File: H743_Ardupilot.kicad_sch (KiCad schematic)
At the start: 8 parts, among them U1 USBLC6-2P6

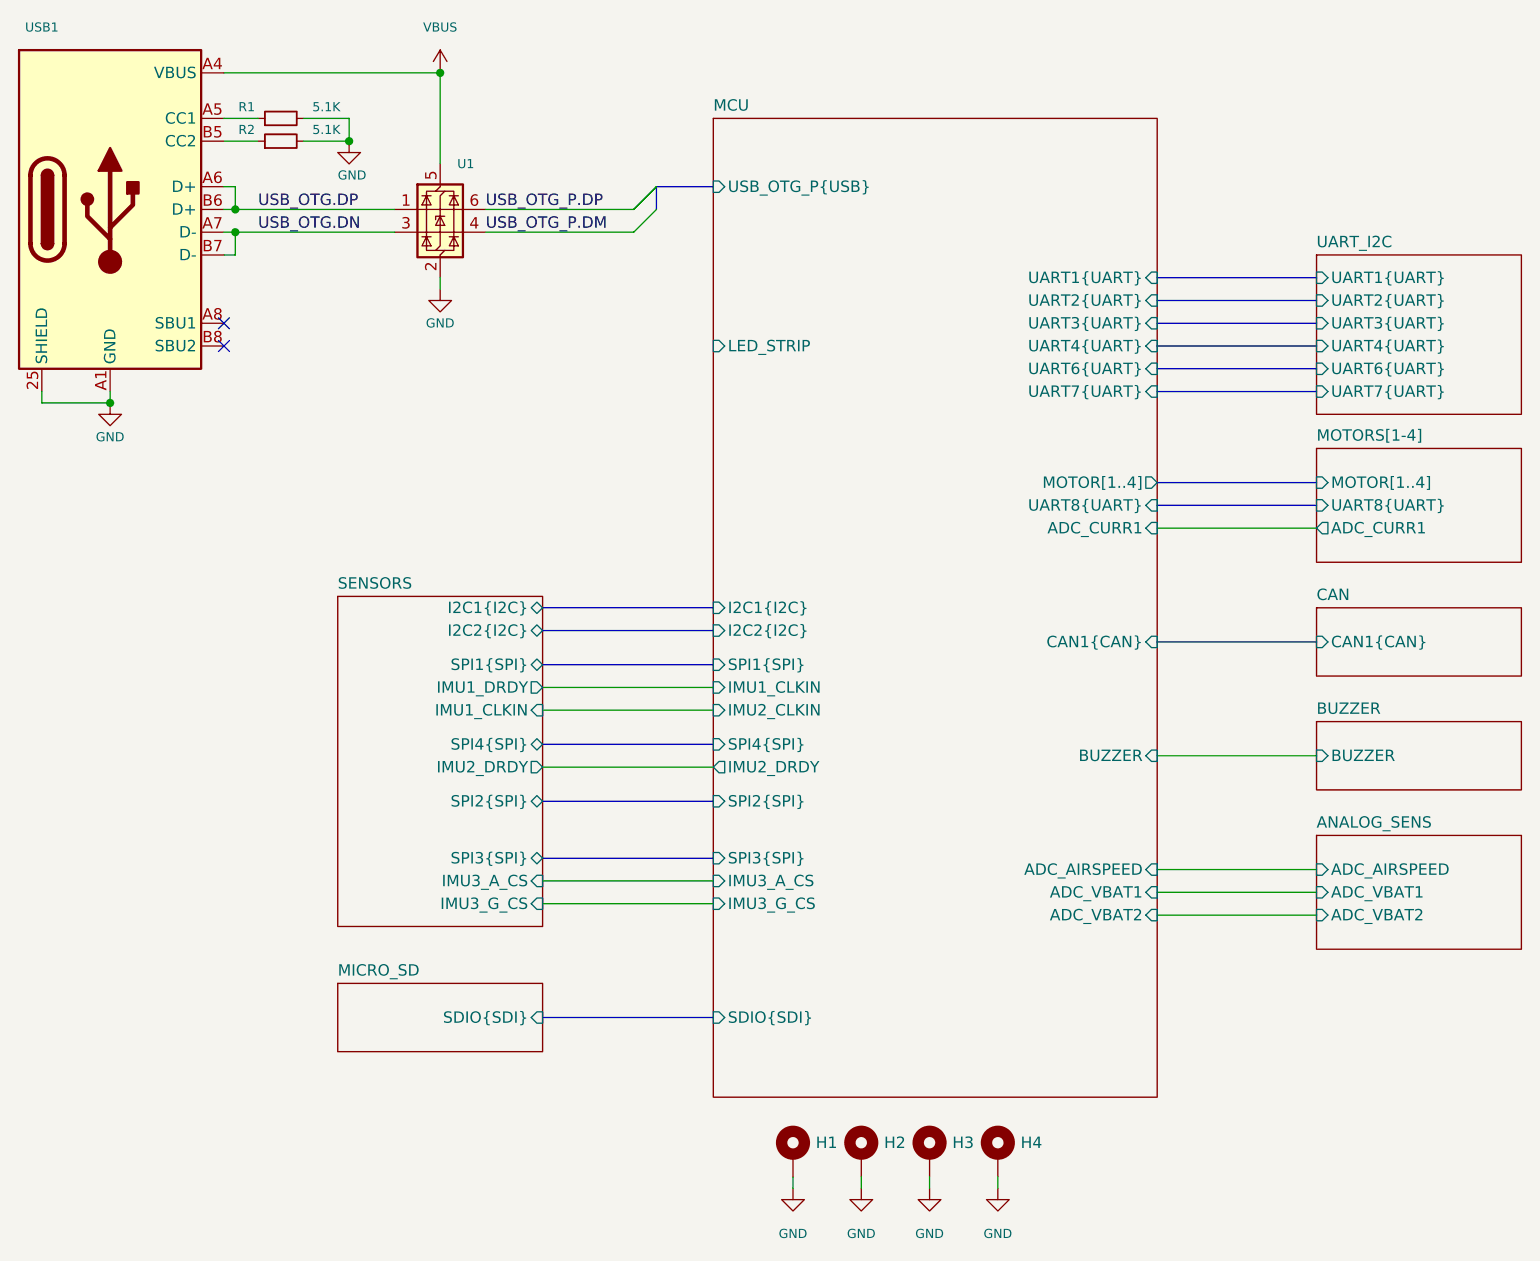
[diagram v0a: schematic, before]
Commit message: re annotate componant globaly
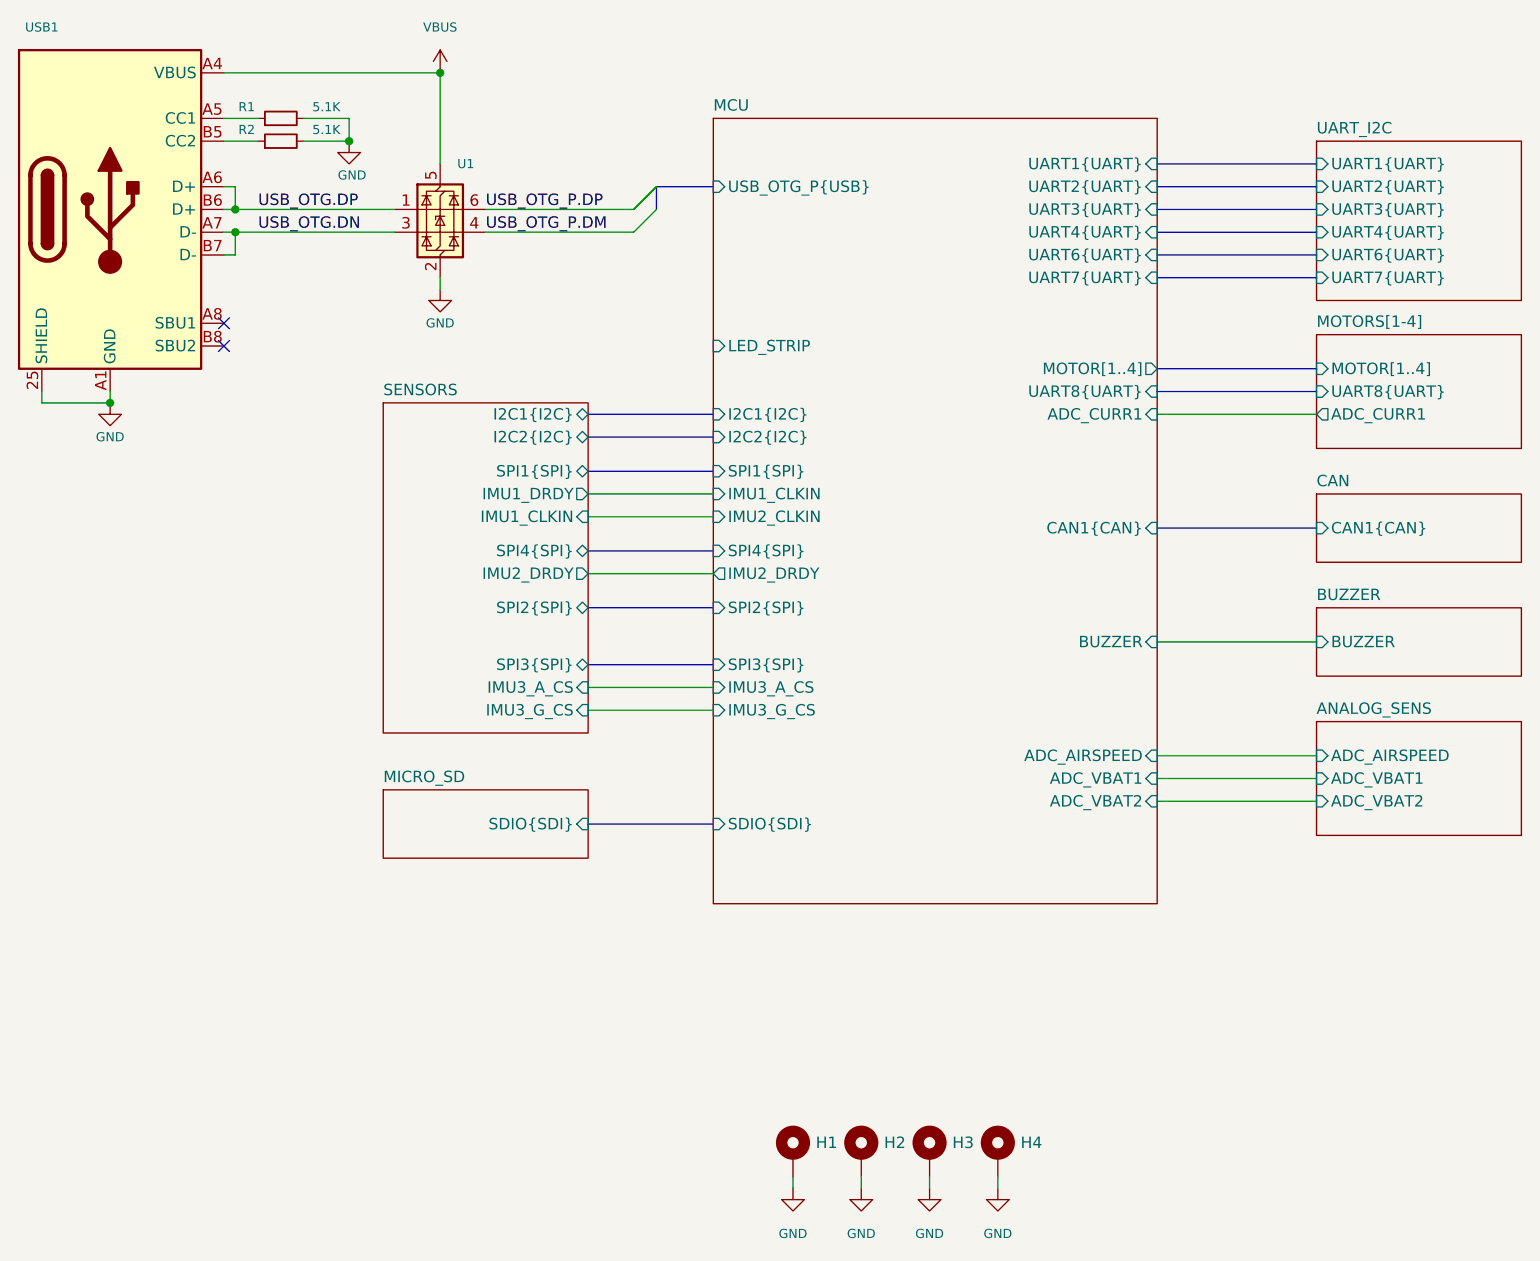
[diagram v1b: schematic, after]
